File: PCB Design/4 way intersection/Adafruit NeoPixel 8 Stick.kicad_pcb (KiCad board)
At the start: 2 copper layers, 33 x 32.5 mm, 9 parts, among them CN1 1X4SMT, CN2 1X4SMT, CN3 1X4SMT, CN4 1X4SMT

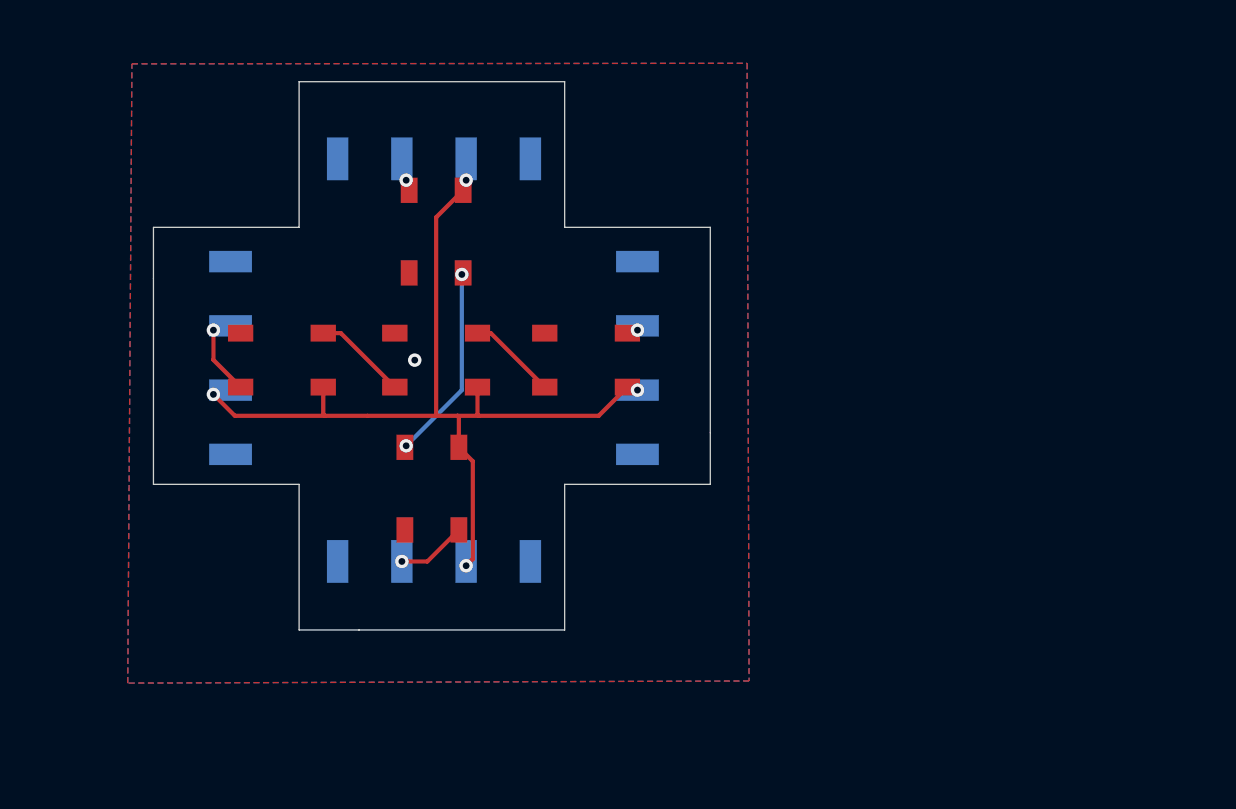
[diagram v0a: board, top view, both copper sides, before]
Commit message: 6 pin
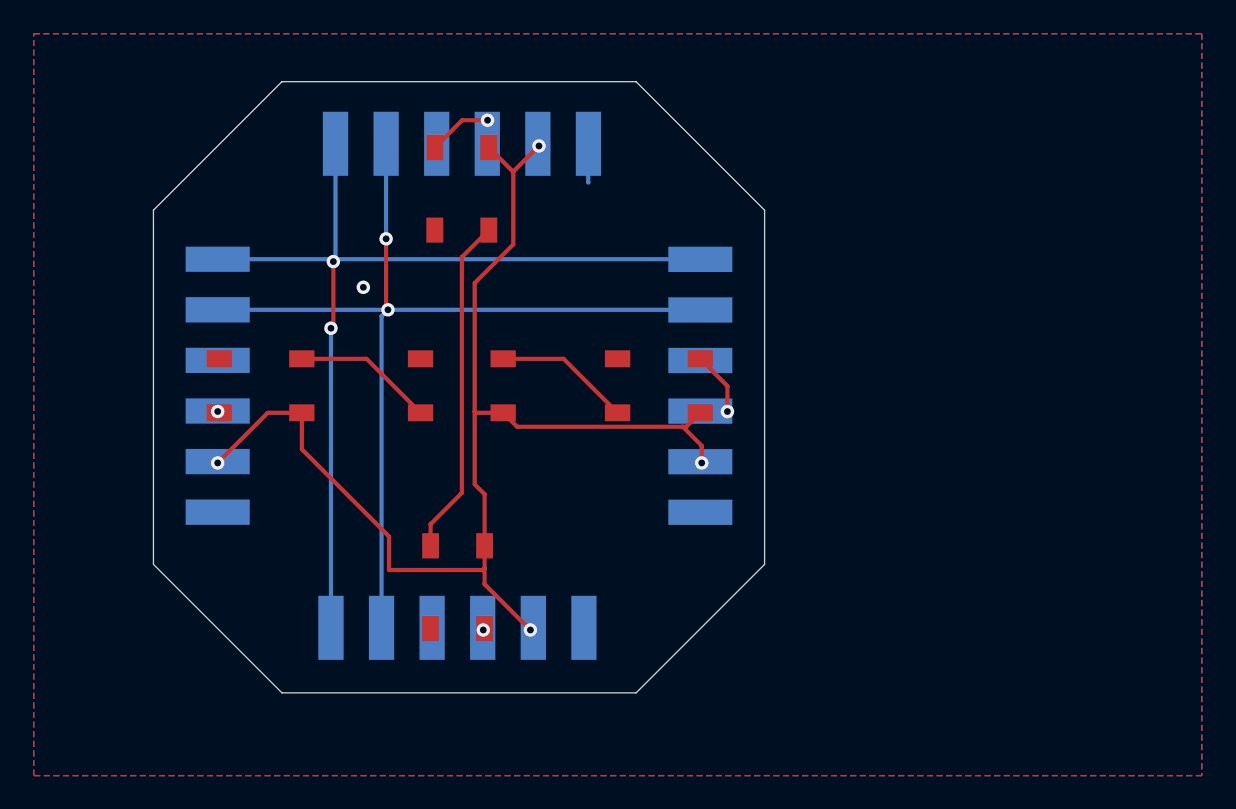
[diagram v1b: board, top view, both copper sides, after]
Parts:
- moved D4 6.04 mm to (140.5, 119.9)
- moved D3 4.58 mm to (152.4, 108.0)
- moved CN1 4.16 mm to (154.2, 108.5)
- moved CN3 3.31 mm to (140.0, 121.7)
- moved D5 2.96 mm to (140.7, 96.3)
- moved CN4 2.81 mm to (141.2, 94.2)
- moved D2 2.16 mm to (140.7, 108.0)
- moved D1 1.98 mm to (128.8, 108.0)
- moved CN2 0.52 mm to (126.9, 107.4)
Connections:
- CN1 pad 1: GND -> Net-(CN1-Pad1)
- CN1 pad 3: +5V -> GND
- CN1 pad 4: GND -> Net-(D3-Pad2)
- CN4 pad 1: GND -> Net-(CN1-Pad1)
- CN4 pad 2: Net-(CN4-Pad2) -> Net-(CN1-Pad2)
- CN4 pad 3: +5V -> GND
- CN4 pad 4: GND -> Net-(CN4-Pad4)
- D3 pad 2: Net-(CN1-Pad2) -> Net-(D3-Pad2)
- D5 pad 2: Net-(CN4-Pad2) -> Net-(CN4-Pad4)
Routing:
- net Net-(CN1-Pad1): track 0.00 -> 57.4 mm, vias 0 -> 2
- net Net-(CN1-Pad2): track 0.00 -> 57.3 mm, vias 1 -> 2
- net +5V: track 52.7 -> 73.8 mm
- net Net-(D4-Pad2): track 11.5 -> 20.2 mm, vias 2 -> 0
- net Net-(CN3-Pad3): track 4.15 -> 0.00 mm
- net Net-(CN2-Pad3): track 4.05 -> 0.00 mm
- net Net-(D3-Pad2): track 0.00 -> 3.79 mm, vias 0 -> 1
- net Net-(CN4-Pad4): track 0.00 -> 3.79 mm, vias 0 -> 1
- net Net-(D2-Pad2): track 5.32 -> 8.11 mm
- net Net-(D1-Pad2): track 5.57 -> 8.36 mm
- net GND: track 0.00 -> 2.17 mm
- net Net-(CN4-Pad2): vias 1 -> 0
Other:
- board size 33 x 32.5 mm -> 36.2 x 36.2 mm
- board text removed: "4-7VDC"
- board text removed: "DOUT"
- board text removed: "GND"
